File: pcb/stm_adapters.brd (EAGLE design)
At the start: 71.6 x 74.9 mm, 65 parts, among them IC1 STM32F405RGT, IC2 STM32F303CBT, IC3 STM32F303x6/x8, IC5 TL431, J1 BUTTON-FSM14JRT, J2 BUTTON-FSM14JRT, J3 BUTTON-FSM14JRT, Q11 32.7680kHz, Q21 32.7680kHz

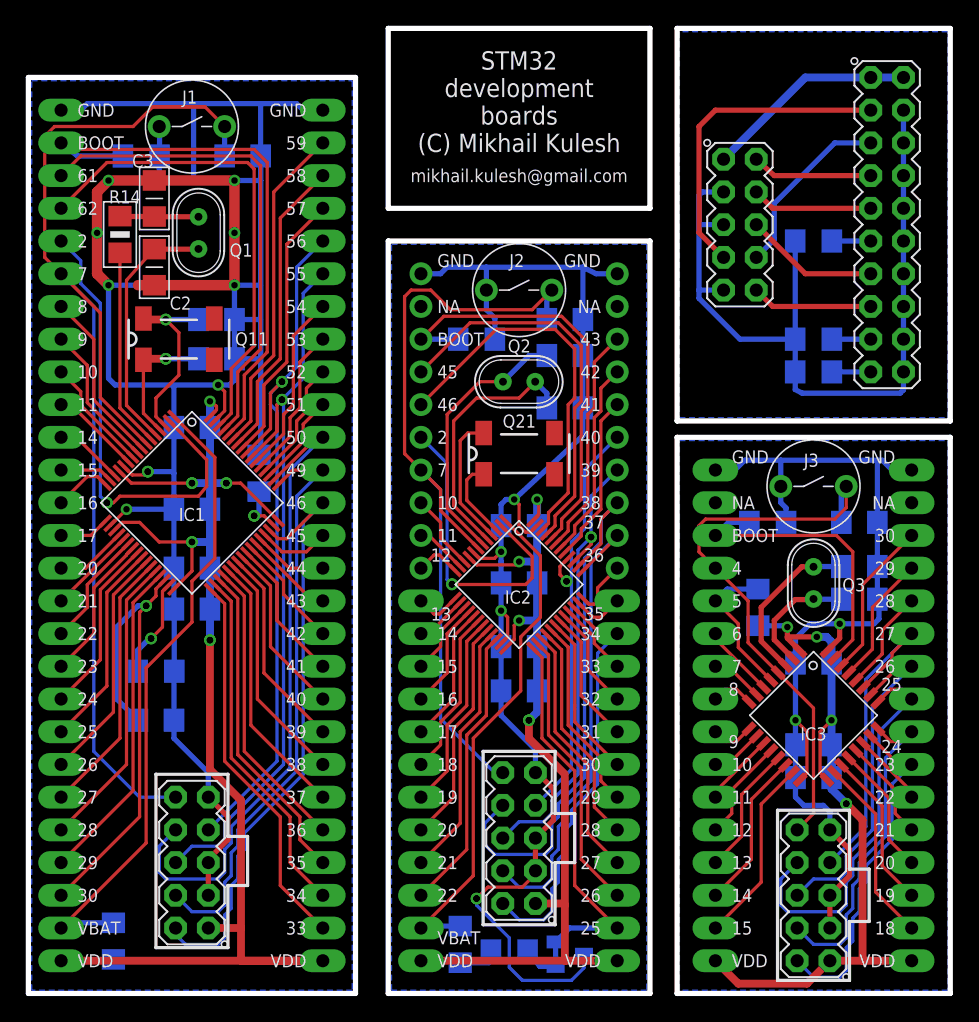
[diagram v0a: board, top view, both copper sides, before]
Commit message: Added version 2 of the boards
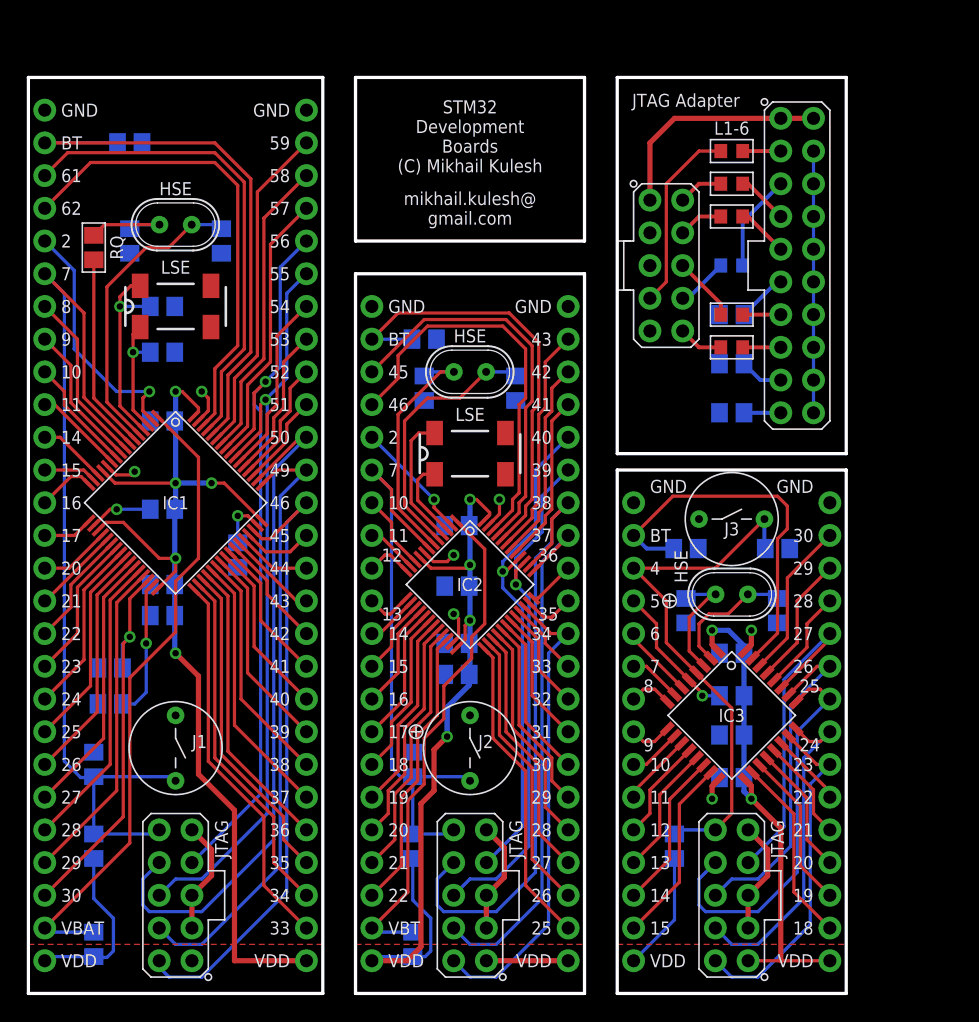
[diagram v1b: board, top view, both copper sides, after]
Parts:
- removed IC5: TL431, MyComponents:SOT-23
- removed R14: 220, rcl:R1206
- removed R2, R3: 0K, rcl:R1206
- removed SV17, SV18: (no value), con-lstb:MA10-1
- added L1, L2, L3, L4, L5, L6: (no value), MyComponents:L0603
- added R10, R32: 10K, MyComponents:R0805
- added R20, R30: 0, MyComponents:R0805
- added RQ: 220, MyComponents:R0805
- added SV19: (no value), MyComponents:MA09-1-NO-PL
- added SV5: (no value), MyComponents:MA07-1-NO-PL
- C1: value 4.7uF -> P30; device rcl:C1206 -> MyComponents:C0805
- C11, C14, C15, C2, C22, C3, C32: device rcl:C1206 -> MyComponents:C0805
- C12, C13, C16, C19, C21, C23, C27, C28, C30, C31, C35: value 100nF -> 0.1uF; device rcl:C1206 -> MyComponents:C0805
- C24, C25, C33, C34: value 10pF -> 12pF; device rcl:C1206 -> MyComponents:C0805
- Q1, Q2, Q3: value (none) -> HSE
- Q11, Q21: value 32.7680kHz -> LSE; device crystal:MC-306 -> MyComponents:MC-306
- R11: value 0K -> 0; device rcl:R1206 -> MyComponents:R0805
- R12: value 0K -> P31; device rcl:R1206 -> MyComponents:R0805
- R13: value 0K -> P47; device rcl:R1206 -> MyComponents:R0805
- R15, R22, R31, R40, R41, R42: device rcl:R1206 -> MyComponents:R0805
- R21: value 330 -> 10K; device rcl:R1206 -> MyComponents:R0805
- SV1, SV3: device con-lstb:MA20-1 -> MyComponents:MA20-1-NO-PL
- SV10, SV11: device con-lstb:MA08-1 -> MyComponents:MA08-1-NO-PL
- SV12: device con-lstb:MA08-1 -> MyComponents:MA09-1-NO-PL
- SV13, SV14, SV15, SV4: device con-lstb:MA05-2 -> MyComponents:MA05-2
- SV16: device con-lstb:MA10-2 -> MyComponents:MA10-2
- SV2, SV8: device con-lstb:MA07-1 -> MyComponents:MA07-1-NO-PL
- SV6, SV7: device con-lstb:MA12-1 -> MyComponents:MA12-1-NO-PL
- SV9: device con-lstb:MA08-1 -> MyComponents:MA07-1-NO-PL
- moved C19 48.6 mm to (5.08, 17.8), turned to 270 degrees
- moved J1 48.3 mm to (11.4, 19.1), turned to 270 degrees
- moved R21 48.0 mm to (30.7, 50.8), turned to 180 degrees
- moved SV12 43.4 mm to (26.7, 43.2), turned to 270 degrees
- moved R22 39.7 mm to (29.8, 11.4), turned to 90 degrees
- moved C28 36.5 mm to (29.8, 17.8), turned to 270 degrees
- moved J2 35.8 mm to (34.3, 19.1), turned to 270 degrees
- moved C34 13.9 mm to (51.1, 29.7), turned to 90 degrees
- moved C25 11.2 mm to (30.7, 47.0), turned to 90 degrees
- moved SV9 8.98 mm to (62.2, 30.5), turned to 90 degrees
- moved R40 8.54 mm to (54.6, 52.7)
- moved SV16 7.67 mm to (59.7, 56.5)
- moved C32 7.16 mm to (54.6, 20.1)
- moved R42 7.10 mm to (54.6, 45.1)
- moved C30 6.84 mm to (54.6, 16.8)
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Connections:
- net N$64 renamed ACAP1
- net N$65 renamed ACAP2
- new net N$10: L6.2, SV16.15
- new net N$11: L5.2, SV16.13
- new net N$13: L4.2, SV16.9
- new net N$24: L3.2, SV16.7
- new net N$29: L2.2, SV16.5
- new net N$36: L1.2, SV16.3
- net AD_RST: now also L6.1; no longer SV16.15
- net AD_TCK: now also L4.1; no longer SV16.9
- net AD_TDI: now also L2.1; no longer SV16.5
- net AD_TDO: now also L5.1; no longer SV16.13
- net AD_TMS: now also L3.1; no longer SV16.7
- net AD_TRST: now also L1.1; no longer SV16.3
- net ARST: now also R10.1
- net AVDD: now also R10.2
- net AVSS: now also SV4.5
- net B10: now also SV12.7; no longer SV17.8
- net B11: now also SV12.8; no longer SV17.9
- net B12: now also SV12.9; no longer SV17.10
- net B2: now also SV12.5; no longer SV17.6
- net B36: now also SV19.1; no longer SV18.1
- net B41: now also SV19.6; no longer SV18.6
- net B42: now also SV19.7; no longer SV18.7
- net B43: now also SV19.8; no longer SV18.8
- net B45: now also SV12.3; no longer SV17.4
- net B46: now also SV12.4; no longer SV17.5
- net BBAT: now also R20.1; no longer R2.1
- net BBOOT: now also R21.1, SV12.2; no longer R22.1, SV17.3
- net BRST: now also R22.2, SV12.6; no longer SV17.7
- net BTCK: now also SV19.2; no longer SV18.2
- net BTDI: now also SV19.3; no longer SV18.3
- net BTDO: now also SV19.4; no longer SV18.4
- net BTRST: now also SV19.5; no longer SV18.5
- net BVDD: now also R20.2, R22.1; no longer R2.2, R21.2
- net BVREF: no longer IC5.1, IC5.2, R21.1
- net BVSS: now also R21.2, SV12.1, SV19.9; no longer IC5.3, R22.2, SV17.1, SV18.10
- net E28: now also SV9.4; no longer SV12.4
- net E29: now also SV9.5; no longer SV12.5
- net E30: now also SV9.6; no longer SV12.6
- net E6: now also SV5.5; no longer SV9.6
- net E7: now also SV5.6; no longer SV9.7
- net E8: now also SV5.7; no longer SV9.8
- net EBOOT: now also SV5.2; no longer SV9.3
- net ERST: now also R32.2, SV5.3; no longer SV9.4
- net ETDI: now also SV9.1; no longer SV12.1
- net ETDO: now also SV9.2; no longer SV12.2
- net ETRST: now also SV9.3; no longer SV12.3
- net EVDD: now also R30.2, R32.1; no longer R3.2
- net EVDDA: now also R30.1, SV5.4; no longer R3.1, SV9.5
- net EVSS: now also SV5.1, SV9.7; no longer SV12.8, SV9.1
- net N$69: now also Q11.1; no longer Q11.4
- net N$70: now also Q11.4; no longer Q11.1
- net N$72: now also RQ.2; no longer R14.2
- net N$78: now also RQ.1; no longer R14.1
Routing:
- net AVSS: track 215.1 -> 19.1 mm, vias 10 -> 3
- net BVSS: track 103.8 -> 16.6 mm, vias 5 -> 3
- net EVSS: track 73.8 -> 12.4 mm
- net AD_VSS: track 64.4 -> 20.3 mm
- net ARST: track 90.9 -> 73.4 mm
- net BRST: track 63.7 -> 46.4 mm
- net A2: track 36.4 -> 19.3 mm
- net AVDD: track 108.6 -> 92.9 mm
- net EVDD: track 62.9 -> 47.7 mm, vias 4 -> 2
- net B2: track 24.0 -> 9.40 mm
- net AD_TDI: track 14.2 -> 4.01 mm
- net AD_TRST: track 24.8 -> 14.7 mm
- net BVREF: track 34.3 -> 24.4 mm
- net ACAP: track 38.7 -> 30.5 mm
- net N$29: track 0.00 -> 7.58 mm
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- added copper zone on layer 1, net AVDD
- added copper zone on layer 1, net BVDD
- added copper zone on layer 1, net EVDD
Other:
- board size 71.6 x 74.9 mm -> 63.5 x 71.1 mm
- board text added: "BT"
- board text added: "JTAG Adapter"
- board text added: "L1-6"
- board text added: "STM32 Development Boards (C) Mikhail Kulesh"
- board text added: "VBT"
- board text added: "mikhail.kulesh@ gmail.com"
- board text removed: "BOOT"
- board text removed: "NA"
- board text removed: "STM32 development boards (C) Mikhail Kulesh"
- board text removed: "mikhail.kulesh@gmail.com"
